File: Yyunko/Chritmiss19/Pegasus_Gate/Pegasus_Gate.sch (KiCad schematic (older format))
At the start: 23 parts, among them U1 WS2811, U2 WS2811, U3 WS2811, U4 WS2811

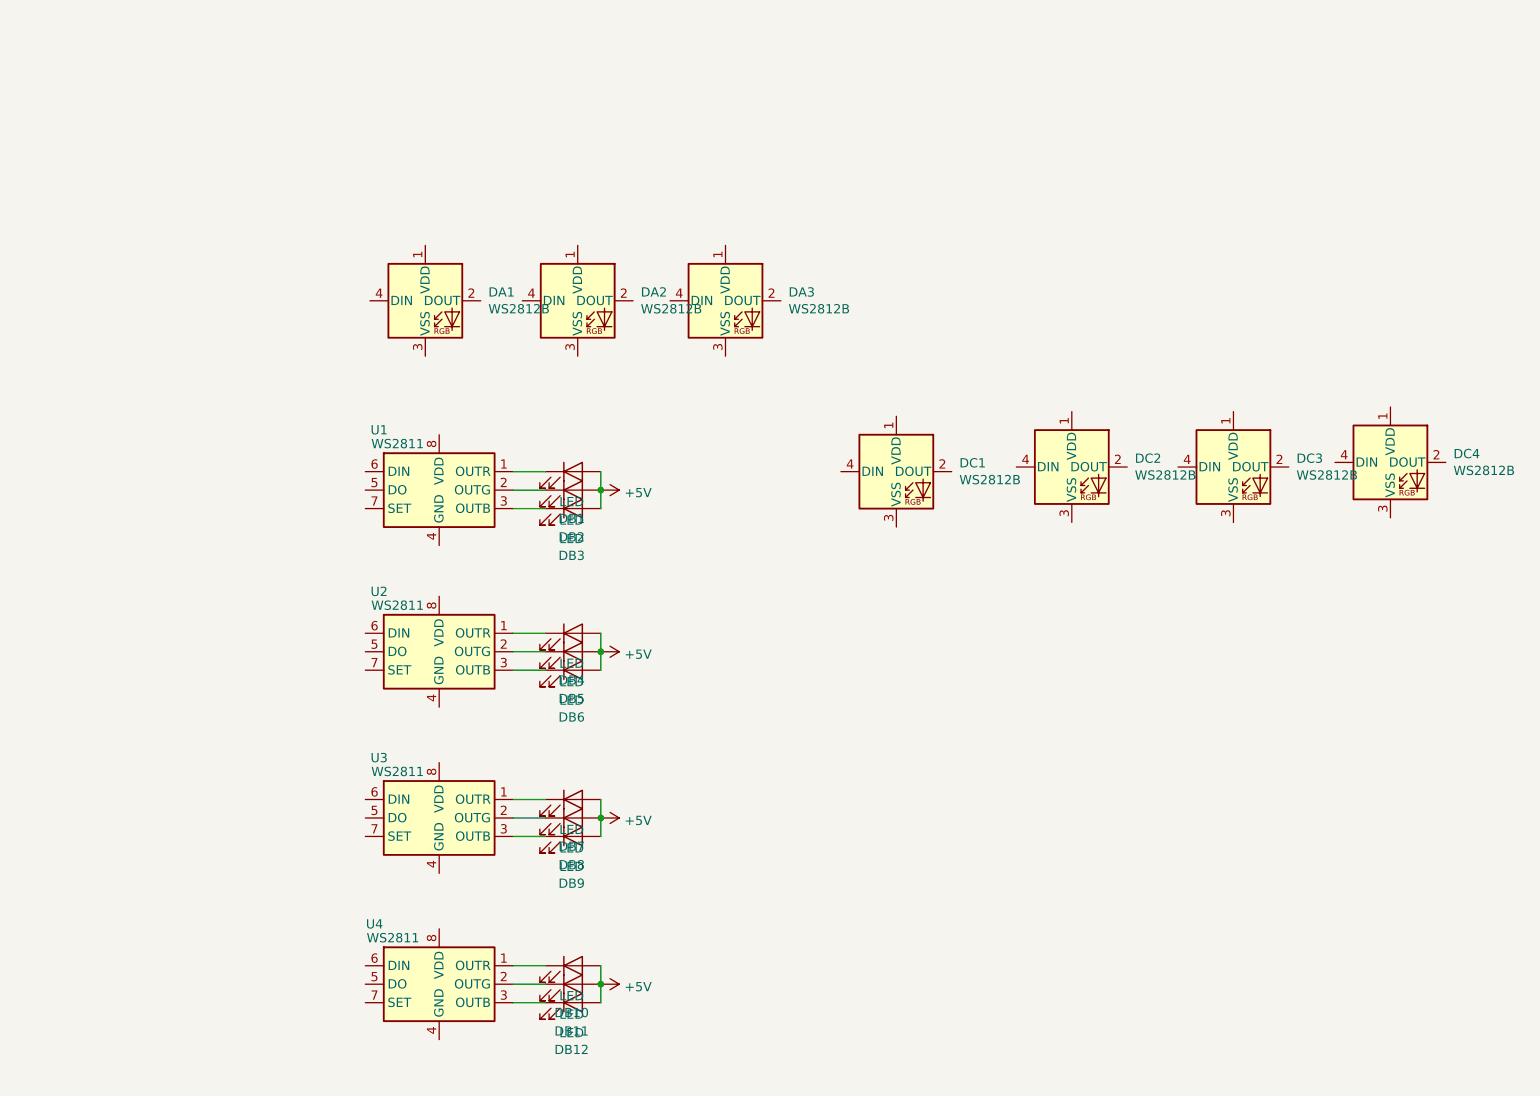
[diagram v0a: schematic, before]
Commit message: Almost sorted all secs out
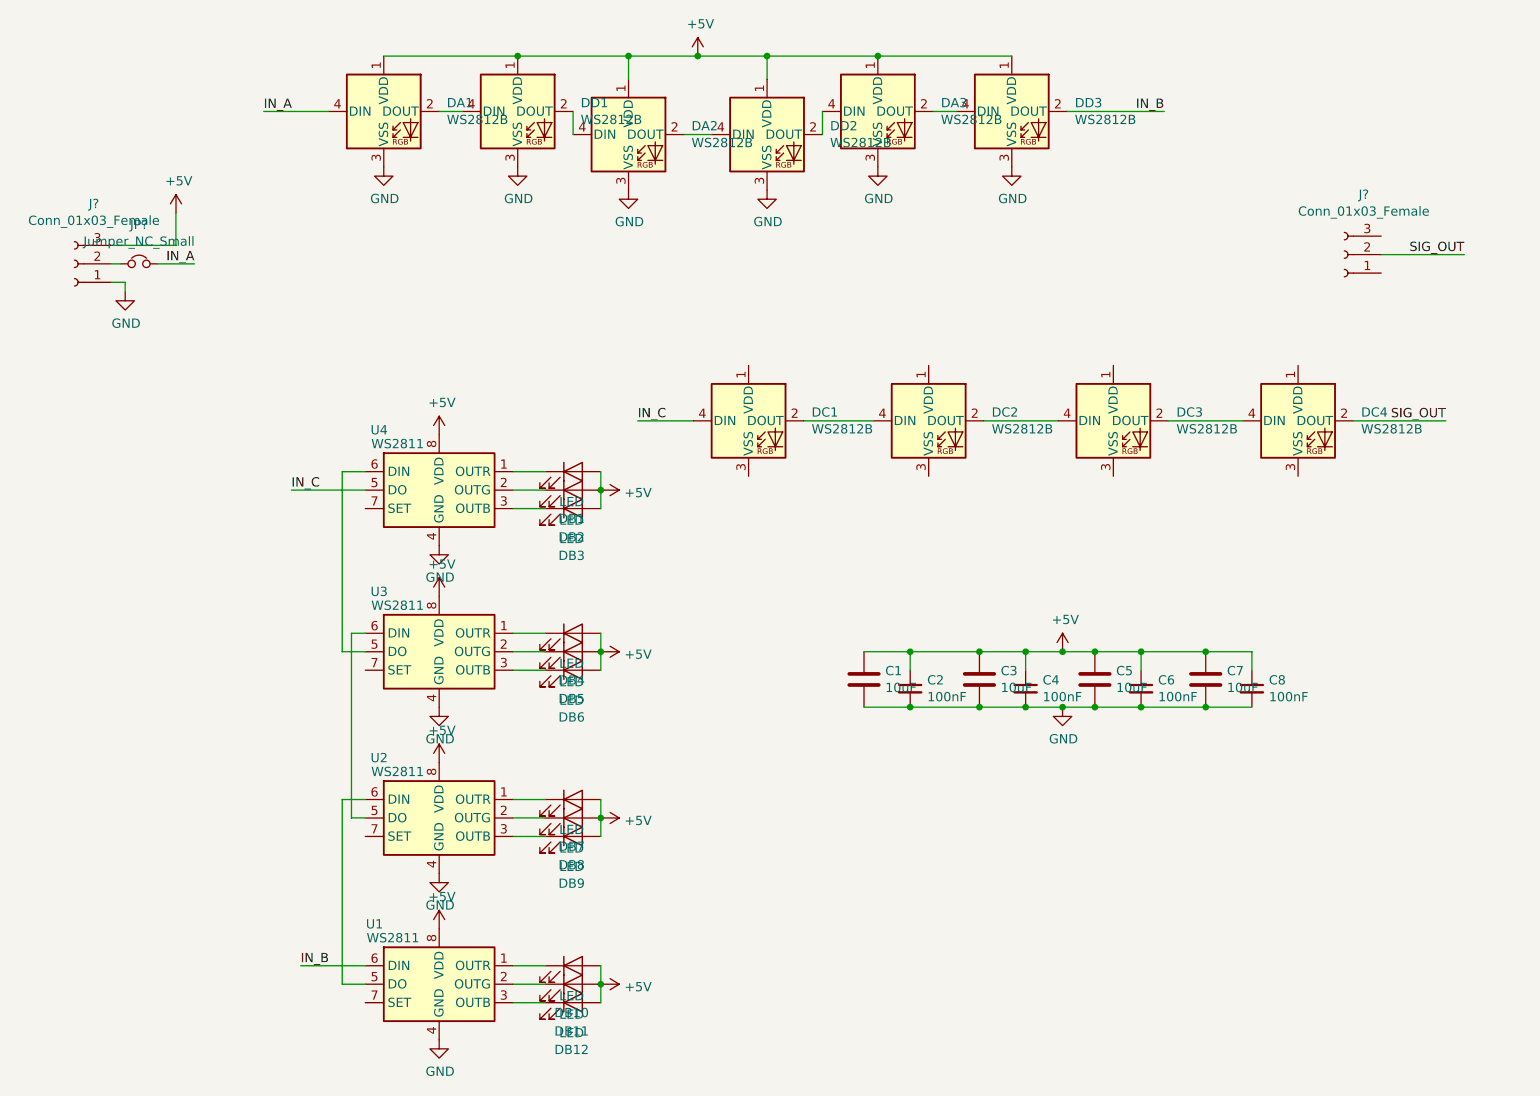
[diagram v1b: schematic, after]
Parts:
- added C1, C3, C5, C7: 10uF, Capacitor_SMD:C_0805_2012Metric, symbol Device:C
- added C2, C4, C6, C8: 100nF, Capacitor_SMD:C_0805_2012Metric, symbol Device:C_Small
- added DD1, DD2, DD3: WS2812B, Local:IN-PI42TAS, symbol LED:WS2812B
- added J? (x2): Conn_01x03_Female, Connector_PinHeader_2.00mm:PinHeader_1x03_P2.00mm_Vertical, symbol Connector:Conn_01x03_Female
- added JP?: Jumper_NC_Small, Jumper:SolderJumper-2_P1.3mm_Bridged_Pad1.0x1.5mm, symbol Device:Jumper_NC_Small
- renumbered U4 to U1, U3 to U2, U2 to U3, U1 to U4
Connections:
- net +5V: now also DA1.1 (VDD), DA2.1 (VDD), DA3.1 (VDD), U1.8 (VDD), U2.8 (VDD), U3.8 (VDD), U4.8 (VDD), C1.1, C2.1, C3.1, C4.1, C5.1, C6.1, C7.1, C8.1, DD1.1 (VDD), DD2.1 (VDD), DD3.1 (VDD), J?.3 (Pin_3)
- net at DA1.2 (DOUT): now also DD1.4 (DIN)
- net GND: now reaches DA1.3 (VSS)
- net GND: now also DA2.3 (VSS), DA3.3 (VSS), U1.4 (GND), U2.4 (GND), U3.4 (GND), U4.4 (GND), C1.2, C2.2, C3.2, C4.2, C5.2, C6.2, C7.2, C8.2, DD1.3 (VSS), DD2.3 (VSS), DD3.3 (VSS), J?.1 (Pin_1)
- net IN_A: now reaches DA1.4 (DIN)
- net IN_A: now also JP?.2
- net at DA2.2 (DOUT): now also DD2.4 (DIN)
- net at DA2.4 (DIN): now also DD1.2 (DOUT)
- net at DA3.2 (DOUT): now also DD3.4 (DIN)
- net at DA3.4 (DIN): now also DD2.2 (DOUT)
- net IN_C: now reaches U4.5 (DO)
- net IN_C: now also DC1.4 (DIN)
- net at U4.6 (DIN): now also U3.5 (DO)
- net at U3.6 (DIN): now also U2.5 (DO)
- net at U2.6 (DIN): now also U1.5 (DO)
- net IN_B: now reaches U1.6 (DIN)
- net IN_B: now also DD3.2 (DOUT)
- net at DC1.2 (DOUT): now also DC2.4 (DIN)
- net at DC2.2 (DOUT): now also DC3.4 (DIN)
- net at DC3.2 (DOUT): now also DC4.4 (DIN)
- net SIG_OUT: now reaches DC4.2 (DOUT)
- net SIG_OUT: now also J?.2 (Pin_2)
- new net: J?.2 (Pin_2), JP?.1
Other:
- moved on the sheet: DA1, DA2, DA3, DC1, DC2, DC3, DC4
